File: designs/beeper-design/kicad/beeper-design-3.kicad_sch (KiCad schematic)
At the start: 22 parts, among them U14 EVPBB4A9B000, U15 EVPBB4A9B000, U16 EVPBB4A9B000, U4 DA7212-01UM2, U9 LSM6DSV16BX

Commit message: exported to Kicad, fixed Kicad, exported gerbers
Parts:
- removed C26: 1u, beeper-design:Pkg0201_9, symbol my_capacitor_4
- removed C27: 100n, beeper-design:Pkg0201_12, symbol my_capacitor_5
- removed C28: 1u, beeper-design:Pkg0201_4, symbol my_capacitor_1
- removed C29: 1u, beeper-design:Pkg0201_27, symbol my_capacitor_13
- removed C30: 1u, beeper-design:Pkg0201_45, symbol my_capacitor_23
- removed C31: 1u, beeper-design:Pkg0201_1, symbol my_capacitor
- removed C32: 1u, beeper-design:Pkg0201_20, symbol my_capacitor_10
- removed C37: 1u, beeper-design:Pkg0201_32, symbol my_capacitor_16
- removed C38: 1u, beeper-design:Pkg0201_38, symbol my_capacitor_19
- removed C39: 1u, beeper-design:Pkg0201_15, symbol my_capacitor_7
- removed C42: 100n, beeper-design:Pkg0201, symbol my_capacitor_26
- removed C43: 100n, beeper-design:Pkg0201_7, symbol my_capacitor_3
- removed R10: 0R, beeper-design:Pkg0201_23, symbol my_resistor_9
- removed R9: 0R, beeper-design:Pkg0201_17, symbol my_resistor_6
- removed U4: DA7212-01UM2, beeper-design:LP_6, symbol component_2
- added C26: 1u, beeper-design:Pkg0201_24, symbol my_capacitor_14
- added C27: 100n, beeper-design:Pkg0201_27, symbol my_capacitor_15
- added C28: 1u, beeper-design:Pkg0201_19, symbol my_capacitor_11
- added C29: 1u, beeper-design:Pkg0201_42, symbol my_capacitor_23
- added C30: 1u, beeper-design:Pkg0201_12, symbol my_capacitor_6
- added C31: 1u, beeper-design:Pkg0201_16, symbol my_capacitor_10
- added C32: 1u, beeper-design:Pkg0201_35, symbol my_capacitor_20
- added C37: 1u, beeper-design:Pkg0201_47, symbol my_capacitor_26
- added C38: 1u, beeper-design:Pkg0201_5, symbol my_capacitor_2
- added C39: 1u, beeper-design:Pkg0201_30, symbol my_capacitor_17
- added C42: 100n, beeper-design:Pkg0201_15, symbol my_capacitor_9
- added C43: 100n, beeper-design:Pkg0201_22, symbol my_capacitor_13
- added R10: 0R, beeper-design:Pkg0201_38, symbol my_resistor_11
- added R9: 0R, beeper-design:Pkg0201_32, symbol my_resistor_8
- added U4: DA7212-01UM2, beeper-design:LP_3, symbol component
- D1: footprint beeper-design:LP -> beeper-design:LP_5
- U14, U15, U16: footprint beeper-design:LP_5 -> beeper-design:LP_2
- U9: footprint beeper-design:LP_4 -> beeper-design:LP_1
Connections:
- net GND: now also C26.1, C27.1, C28.1, C29.1, C30.1, C31.1, C32.1, C37.1, C38.1, C39.1, C42.1, C43.1, U4.B10 (GND_A), U4.B2 (GND_CP)
- net MICBIAS1: now also C37.2, U4.A15 (MICBIAS1)
- net SP_N: now also U4.A13 (SP_N)
- net SP_P: now also U4.B12 (SP_P)
- net VDD1P8: now also C42.2, C43.2
- net VDD1P8P: now also C28.2, U4.B6 (VDD_A)
- net VDD3P0: now also C26.2, C32.2, U4.B14 (VDD_MIC), U4.D10 (VDD_IO)
- net VDDSYS: now also C29.2, U4.A11 (VDD_SP)
- net board-io_clk: now also U4.C17 (MIC1_P)
- net board-io_data: now also U4.B16 (MIC1_N)
- net mcu_sck: now also R10.2
- net mcu_scl: now also R10.1
- net mcu_scl2: now also U4.D8 (SCL)
- net mcu_sda: now also U4.C9 (SDA)
- net mcu_sda2: now also R9.1
- net mcu_sdo: now also R9.2
- new net: C30.2, U4.A9 (VMID)
- new net: C31.2, U4.A7 (DACREF)
- new net: C38.2, U4.A17 (MICBIAS2)
- new net: C39.2, U4.B8 (VREF)
- new net: C27.2, U4.D12 (VDIG)

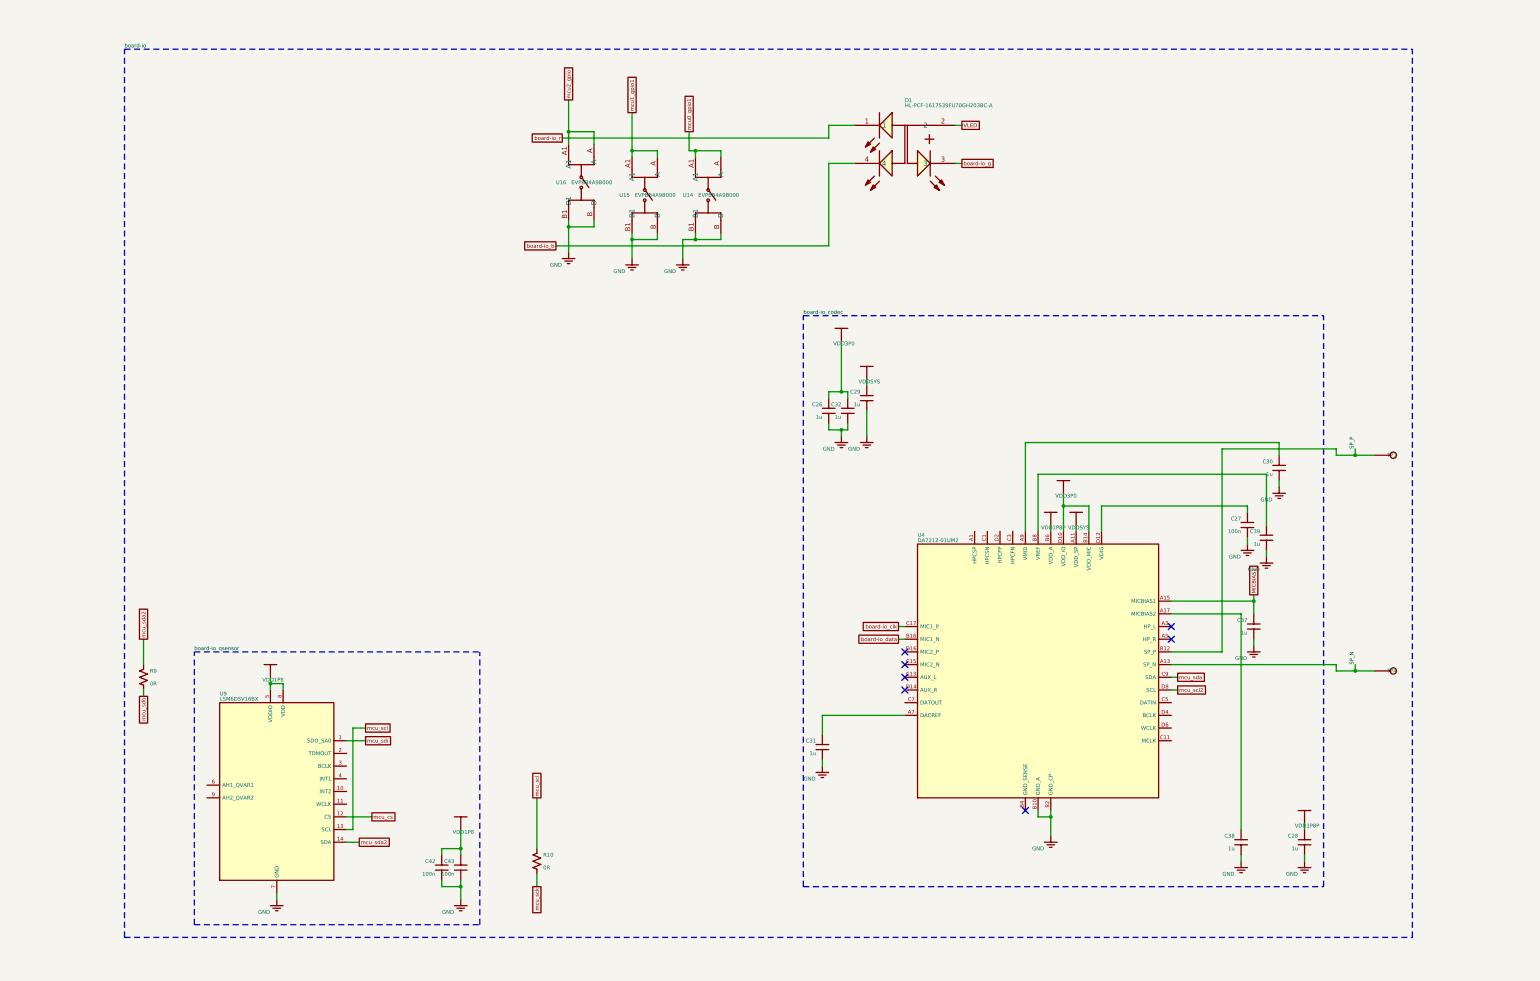
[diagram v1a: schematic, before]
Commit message: latest fully routed version
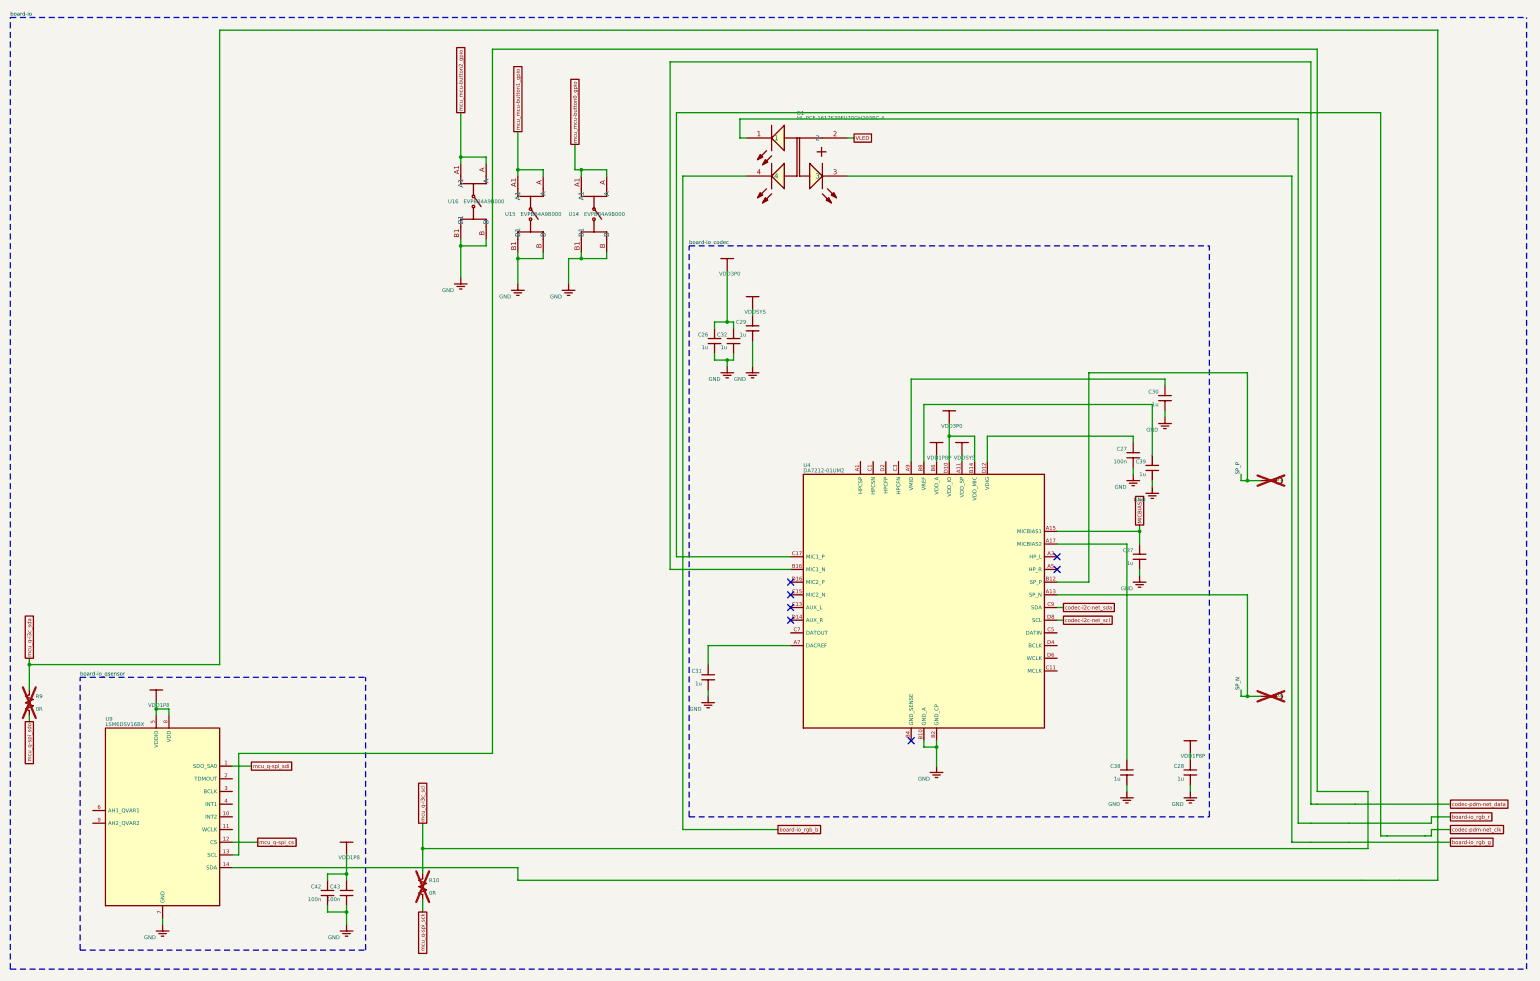
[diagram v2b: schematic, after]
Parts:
- removed C26: 1u, beeper-design:Pkg0201_24, symbol my_capacitor_14
- removed C27: 100n, beeper-design:Pkg0201_27, symbol my_capacitor_15
- removed C28: 1u, beeper-design:Pkg0201_19, symbol my_capacitor_11
- removed C29: 1u, beeper-design:Pkg0201_42, symbol my_capacitor_23
- removed C30: 1u, beeper-design:Pkg0201_12, symbol my_capacitor_6
- removed C31: 1u, beeper-design:Pkg0201_16, symbol my_capacitor_10
- removed C37: 1u, beeper-design:Pkg0201_47, symbol my_capacitor_26
- removed C38: 1u, beeper-design:Pkg0201_5, symbol my_capacitor_2
- removed C39: 1u, beeper-design:Pkg0201_30, symbol my_capacitor_17
- removed C42: 100n, beeper-design:Pkg0201_15, symbol my_capacitor_9
- removed C43: 100n, beeper-design:Pkg0201_22, symbol my_capacitor_13
- removed R10: 0R, beeper-design:Pkg0201_38, symbol my_resistor_11
- removed R9: 0R, beeper-design:Pkg0201_32, symbol my_resistor_8
- added C26: 1u, beeper-design:Pkg0201_7, symbol my_capacitor_4
- added C27: 100n, beeper-design:Pkg0201_24, symbol my_capacitor_13
- added C28: 1u, beeper-design:Pkg0201_12, symbol my_capacitor_6
- added C29: 1u, beeper-design:Pkg0201_46, symbol my_capacitor_26
- added C30: 1u, beeper-design:Pkg0201_33, symbol my_capacitor_19
- added C31: 1u, beeper-design:Pkg0201_43, symbol my_capacitor_25
- added C37: 1u, beeper-design:Pkg0201_10, symbol my_capacitor_5
- added C38: 1u, beeper-design:Pkg0201_21, symbol my_capacitor_12
- added C39: 1u, beeper-design:Pkg0201_20, symbol my_capacitor_11
- added C42: 100n, beeper-design:Pkg0201_14, symbol my_capacitor_8
- added C43: 100n, beeper-design:Pkg0201_26, symbol my_capacitor_14
- added R10: 0R, beeper-design:Pkg0201_17, symbol my_resistor_6
- added R9: 0R, beeper-design:Pkg0201_8, symbol my_resistor_3
- D1: footprint beeper-design:LP_5 -> beeper-design:LP_4
- TP3, TP4: now not fitted; now left out of the parts list
- U14, U15, U16: footprint beeper-design:LP_2 -> beeper-design:LP_1
- U4: footprint beeper-design:LP_3 -> beeper-design:LP_2
- U9: footprint beeper-design:LP_1 -> beeper-design:LP
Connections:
- net GND: now also C26.1, C27.1, C28.1, C29.1, C30.1, C31.1, C37.1, C38.1, C39.1, C42.1, C43.1
- net MICBIAS1: now also C37.2
- net VDD1P8: now also C42.2, C43.2
- net VDD1P8P: now also C28.2
- net VDD3P0: now also C26.2
- net VDDSYS: now also C29.2
- net at U4.A9 (VMID): now also C30.2
- net at U4.A7 (DACREF): now also C31.2
- net at U4.A17 (MICBIAS2): now also C38.2
- net at U4.B8 (VREF): now also C39.2
- net at U4.D12 (VDIG): now also C27.2
- net board-io_b renamed board-io_rgb_b
- net board-io_clk renamed codec-pdm-net_clk
- net board-io_data renamed codec-pdm-net_data
- net board-io_g renamed board-io_rgb_g
- net board-io_r renamed board-io_rgb_r
- net mcu0_gpio1 renamed mcu_mcu-button0_gpio
- net mcu1_gpio1 renamed mcu_mcu-button1_gpio
- net mcu2_gpio renamed mcu_mcu-button2_gpio
- net mcu_cs renamed mcu_q-spi_cs
- net mcu_scl renamed mcu_q-i3c_scl
- net mcu_q-i3c_scl: now also R10.1
- net mcu_scl2 renamed codec-i2c-net_scl
- net mcu_sda renamed codec-i2c-net_sda
- net mcu_sda2 renamed mcu_q-i3c_sda
- net mcu_q-i3c_sda: now also R9.1
- net mcu_sdi renamed mcu_q-spi_sdi
- new net mcu_q-spi_sck: R10.2
- new net mcu_q-spi_sdo: R9.2
